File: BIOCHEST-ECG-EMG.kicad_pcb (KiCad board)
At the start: 4 copper layers, 64 x 38 mm, 29 parts, among them J1 ECG+, J2 ECG-, J3 RLD, J4 EMG+, J5 EMG-, J6 USB_C, SW1 RESET, SW2 BOOT, U1 ADS1293, U10 B0503S-1WR3, U11 MAX17048, U2 ISO7741U, U3 ESP32-S3-MINI-1, U7 TPS7A2033, U8 AP2112K-3.3, U9 BQ24075

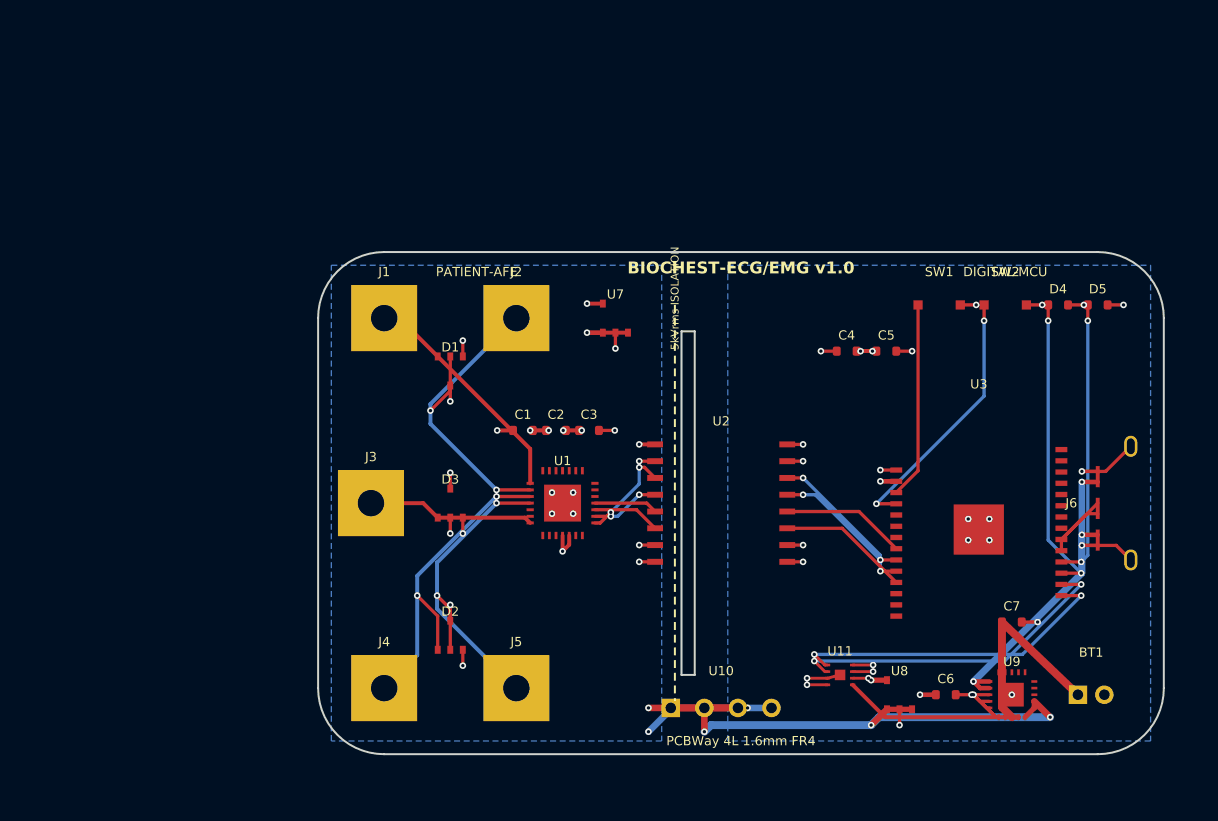
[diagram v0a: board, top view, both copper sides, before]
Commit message: Release v1.1.0: 4-Layer Medical PCBA routing, IPC net classes, 0-DRC validation and Gerber production package
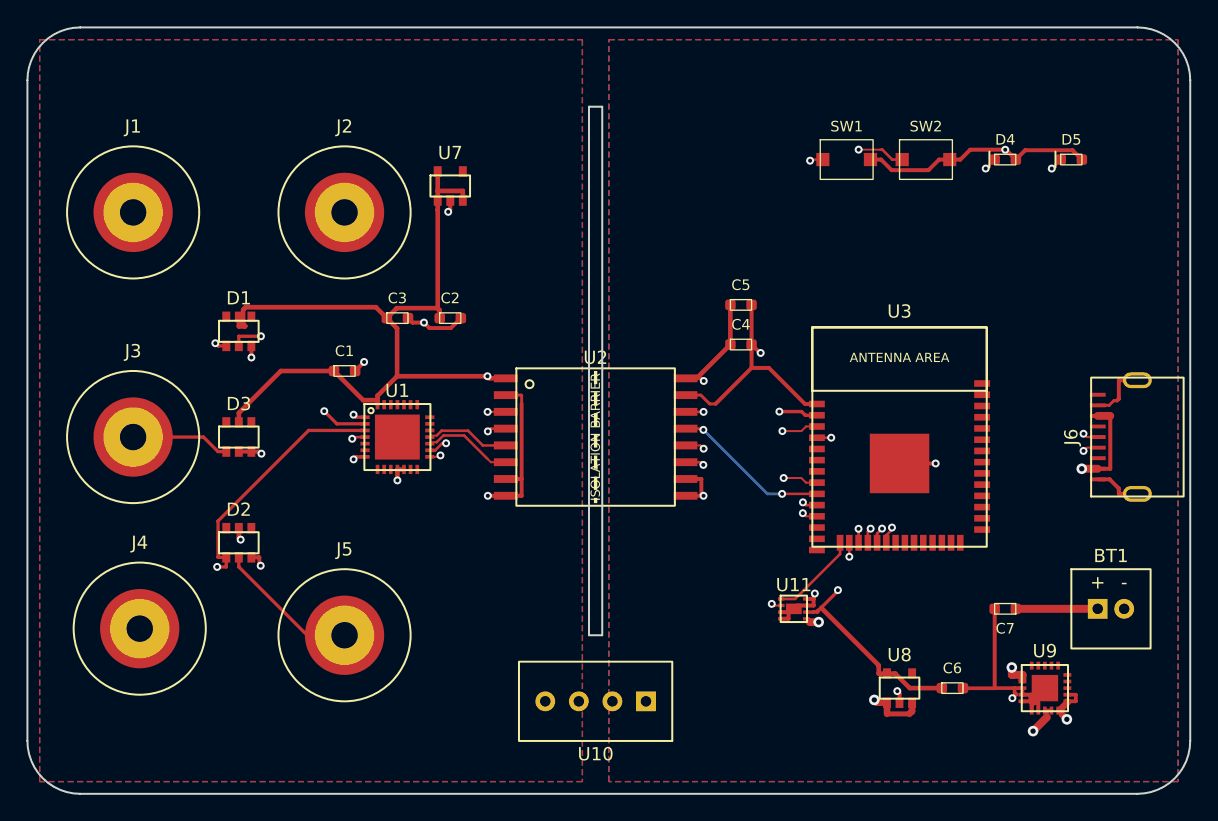
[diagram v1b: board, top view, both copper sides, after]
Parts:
- BT1: value LiPo_800mAh -> VBAT_JST; footprint BIOCHEST:JST_PH_S2B-PH-K-S_1x02_P2.00mm_Horizontal -> JST_PH_S2B-PH-K-S_1x02_P2.00mm_Horizontal
- C1, C2, C4, C6: footprint BIOCHEST:C_0603_1608Metric -> C_0603_1608Metric
- C3: value 100nF_ISO1 -> 100nF_VDD; footprint BIOCHEST:C_0603_1608Metric -> C_0603_1608Metric
- C5: value 10uF_ESP -> 10uF_3V3; footprint BIOCHEST:C_0603_1608Metric -> C_0603_1608Metric
- C7: value 10uF_BAT -> 10uF_VBAT; footprint BIOCHEST:C_0603_1608Metric -> C_0603_1608Metric
- D1, D2, D3: footprint BIOCHEST:TPD2E001_SOT-23 -> TPD2E001_SOT-23
- D4, D5: footprint BIOCHEST:LED_0603_1608Metric -> LED_0603_1608Metric
- J1, J2, J3, J4, J5: footprint BIOCHEST:Snap_Button_Male_10mm -> Snap_Button_Male_10mm
- J6: footprint BIOCHEST:USB_C_Receptacle_16P_SurfaceMount -> USB_C_Receptacle_16P_SurfaceMount
- SW1, SW2: footprint BIOCHEST:SW_Push_SPST_NO_3x4mm -> SW_Push_SPST_NO_3x4mm
- U1: footprint BIOCHEST:ADS1293_WQFN-28_5x5mm -> ADS1293_WQFN-28_5x5mm
- U10: footprint BIOCHEST:B0503S_1WR3_SIP-4 -> B0503S_1WR3_SIP-4
- U11: footprint BIOCHEST:MAX17048_DFN-8_2x2mm -> MAX17048_DFN-8_2x2mm
- U2: footprint BIOCHEST:ISO7741U_SOIC-16W_DWW -> ISO7741U_SOIC-16W_DWW
- U3: footprint BIOCHEST:ESP32-S3-MINI-1 -> ESP32-S3-MINI-1
- U7, U8: footprint BIOCHEST:SOT-23-5 -> SOT-23-5
- U9: footprint BIOCHEST:BQ24075_QFN-20_3.5x3.5mm -> BQ24075_QFN-20_3.5x3.5mm
- moved J1 20.6 mm to (54.0, 78.0)
- moved J4 19.0 mm to (54.5, 109.5)
- moved J3 18.7 mm to (54.0, 95.0)
- moved D2 17.5 mm to (62.0, 103.0)
- moved C3 16.8 mm to (74.0, 86.0)
- moved D3 16.8 mm to (62.0, 95.0)
- moved D1 16.3 mm to (62.0, 87.0)
- moved U7 16.0 mm to (78.0, 76.0)
- moved J2 15.3 mm to (70.0, 78.0)
- moved C1 14.2 mm to (70.0, 90.0)
- moved J5 13.6 mm to (70.0, 110.0)
- moved U1 13.5 mm to (74.0, 95.0)
- moved SW1 13.0 mm to (108.0, 74.0)
- moved SW2 12.5 mm to (114.0, 74.0)
- moved D4 11.7 mm to (120.0, 74.0)
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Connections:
- BT1 pad 2: BAT_PROT_N -> DGND
- U1 pad 28: (no net) -> 3V3_AFE
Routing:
- net DGND: track 49.6 -> 202.5 mm, vias 26 -> 7
- net 3V3_AFE: track 26.6 -> 109.3 mm, vias 11 -> 3
- net AGND: track 20.0 -> 99.6 mm, vias 16 -> 7
- net 3V3_DIG: track 8.40 -> 48.6 mm, vias 7 -> 3
- net LED_ALERT: track 21.2 -> 40.1 mm
- net I2C_SDA: track 24.9 -> 6.71 mm, vias 2 -> 0
- net I2C_SCL: track 25.4 -> 9.17 mm
- net USB_DN: track 4.74 -> 20.7 mm, vias 0 -> 2
- net USB_DP: track 3.56 -> 19.4 mm, vias 0 -> 2
- net VBAT: track 29.0 -> 42.5 mm, vias 0 -> 2
- net RLD_DRV: track 12.7 -> 25.8 mm, vias 0 -> 1
- net LED_STATUS: track 22.8 -> 35.6 mm
- net VBUS: track 38.0 -> 26.2 mm, vias 3 -> 2
- net ESP_EN: track 14.9 -> 25.1 mm, vias 0 -> 2
- net ECG_P: track 17.8 -> 27.3 mm, vias 0 -> 2
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- added copper zone on F.Cu, net AGND
- added copper zone on In2.Cu, net AGND
- added copper zone on F.Cu, net DGND
- added copper zone on In2.Cu, net DGND
- removed copper zone on In2.Cu, net 3V3_AFE
- removed copper zone on In2.Cu, net 3V3_DIG
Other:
- board size 64 x 38 mm -> 88 x 58 mm
- board text removed: "5kVrms ISOLATION"
- board text removed: "BIOCHEST-ECG/EMG v1.0"
- board text removed: "DIGITAL-MCU"
- board text removed: "PATIENT-AFE"
- board text removed: "PCBWay 4L 1.6mm FR4"
